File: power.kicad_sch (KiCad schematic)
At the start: 49 parts, among them J201 -, J202 -, J203 Barrel_Jack_MountingPin, Q201 AOD4185, U101 74HC04, U102 74HC08, U103 74HC32, U201 MP9942GJ

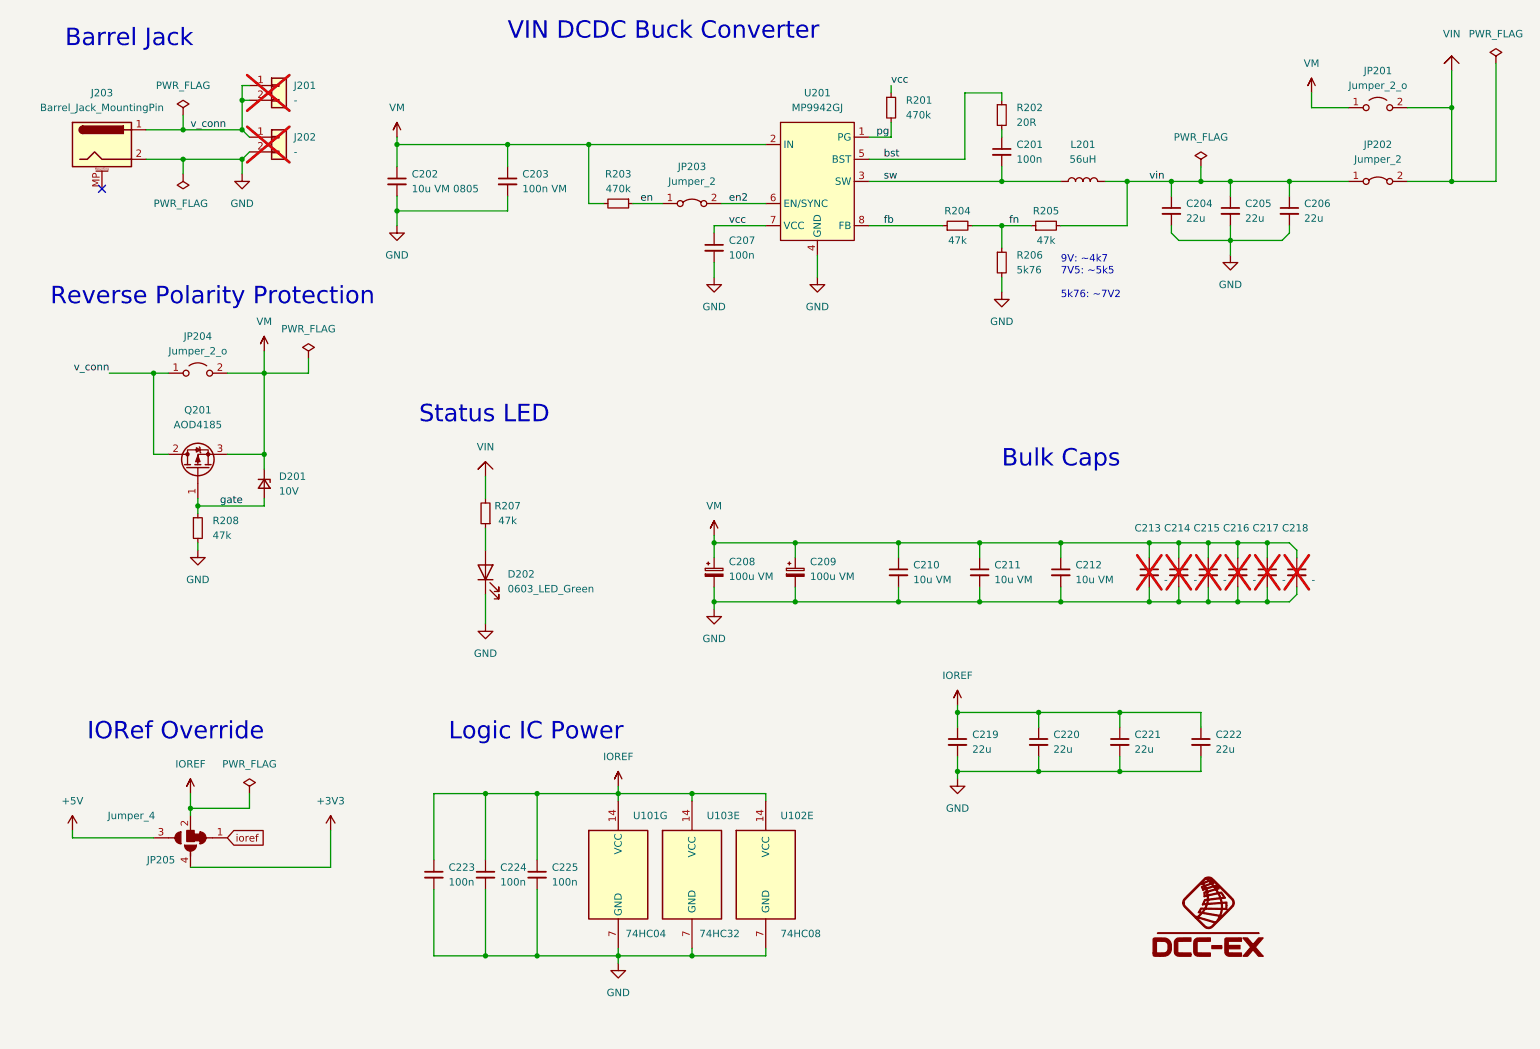
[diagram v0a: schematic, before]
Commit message: Rev A2
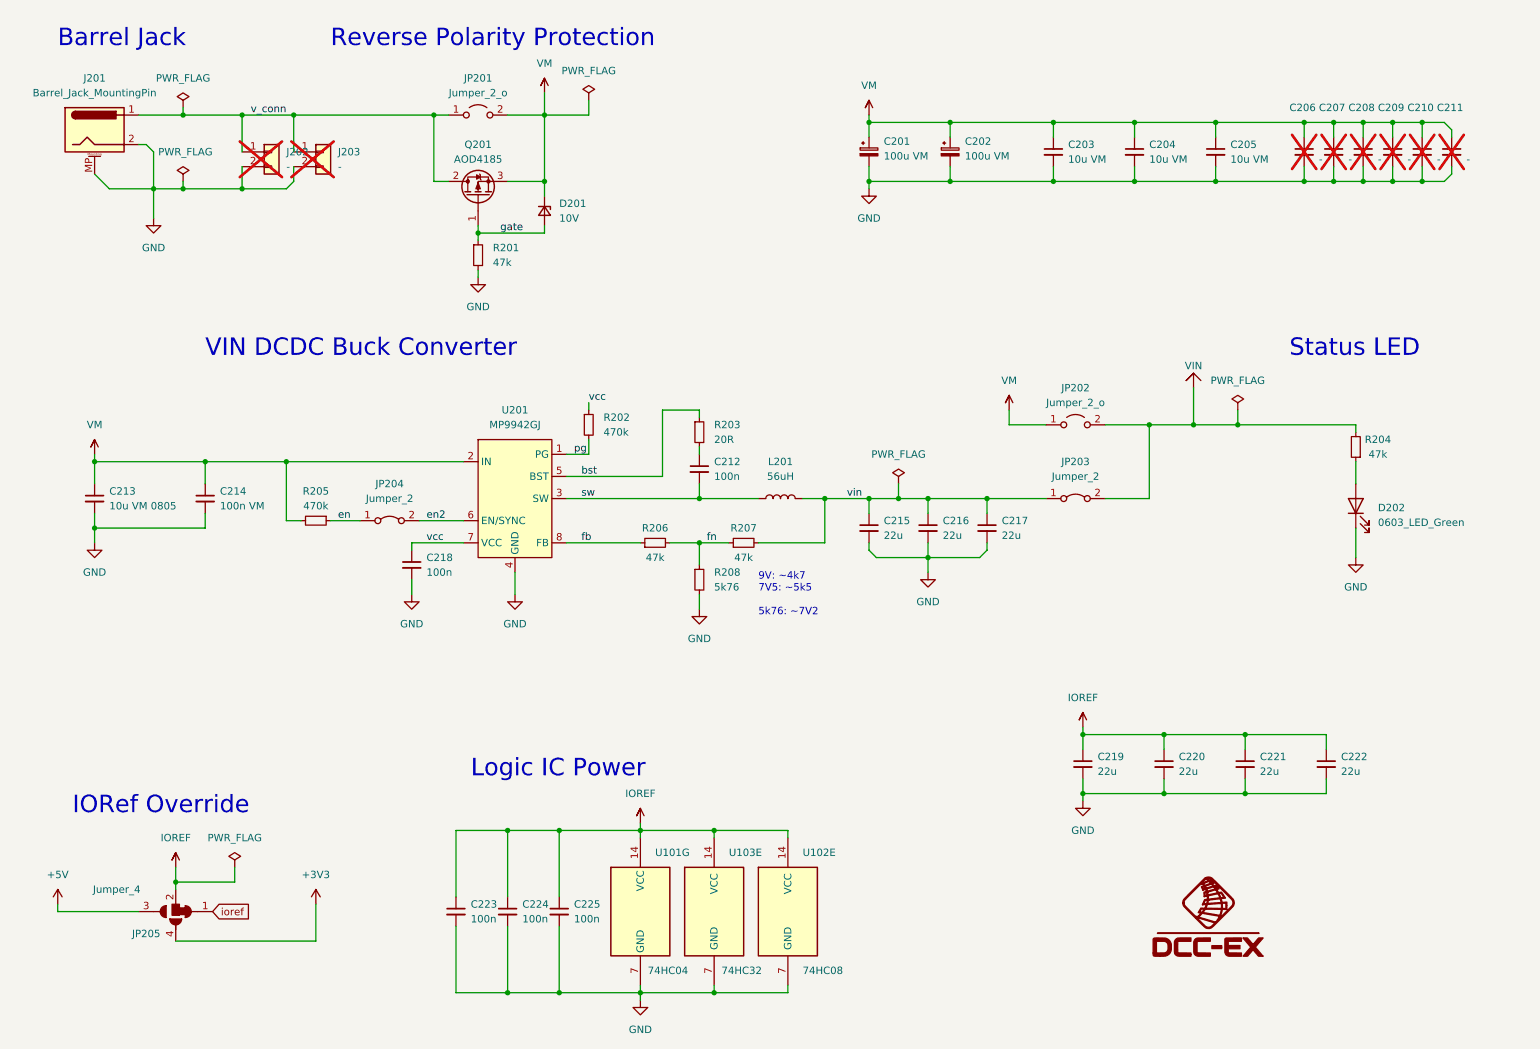
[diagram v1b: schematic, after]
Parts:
- J201: renamed from J203; footprint _my:BarrelJack_2.1mm -> _my:BarrelJack_2.1mm_SMD; LCSC Part # C194407 -> C2936010
- J202: footprint _my:PinHeader_01x03_P2.5mm_Vertical_min -> _my:PinHeader_01x02_P5mm_Vertical_min
- J203: renamed from J201; footprint _my:PinHeader_1x02_P2.54mm_Vertical_min -> _my:PinHeader_1x04_P2.54mm_Vertical_min_1
- JP203: renamed from JP202; footprint Jumper:SolderJumper-2_P1.3mm_Bridged2Bar_RoundedPad1.0x1.5mm -> _my:SolderJumper-2_P1.3mm_Bridged
- JP204: renamed from JP203; footprint Jumper:SolderJumper-2_P1.3mm_Bridged2Bar_RoundedPad1.0x1.5mm -> _my:SolderJumper-2_P1.3mm_Bridged
- renumbered C208 to C201, C209 to C202, C210 to C203, C211 to C204, C212 to C205, C213 to C206, C214 to C207, C215 to C208, C216 to C209, C217 to C210, C218 to C211, C201 to C212, C202 to C213, C203 to C214, C204 to C215, C205 to C216, C206 to C217, C207 to C218, JP204 to JP201, JP201 to JP202, R208 to R201, R201 to R202, R202 to R203, R207 to R204, R203 to R205, R204 to R206, R205 to R207, R206 to R208
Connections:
- net GND: now also J201.MP (MountPin), J203.2 (Pin_2)
- net v_conn: no longer J203.2 (Pin_2)
- no-connect marks 1 -> 0
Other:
- note removed: "Bulk Caps"
- moved on the sheet: C201, C202, C203, C204, C205, C206, C207, C208, C209, C210, C211, C212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
